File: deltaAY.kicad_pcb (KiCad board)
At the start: 2 copper layers, 97 x 61.4 mm, 18 parts, among them J1 SNP, J2 Jack_3.5mm_5pin, U1 М555ЛН1 (SN74LS04), U2 К555ТМ2 (SN74LS74), U3 К555ЛЛ1 (SN74LS32), U4 К555ЛЕ1 (SN74LS02), Y1 3.579545Mhz

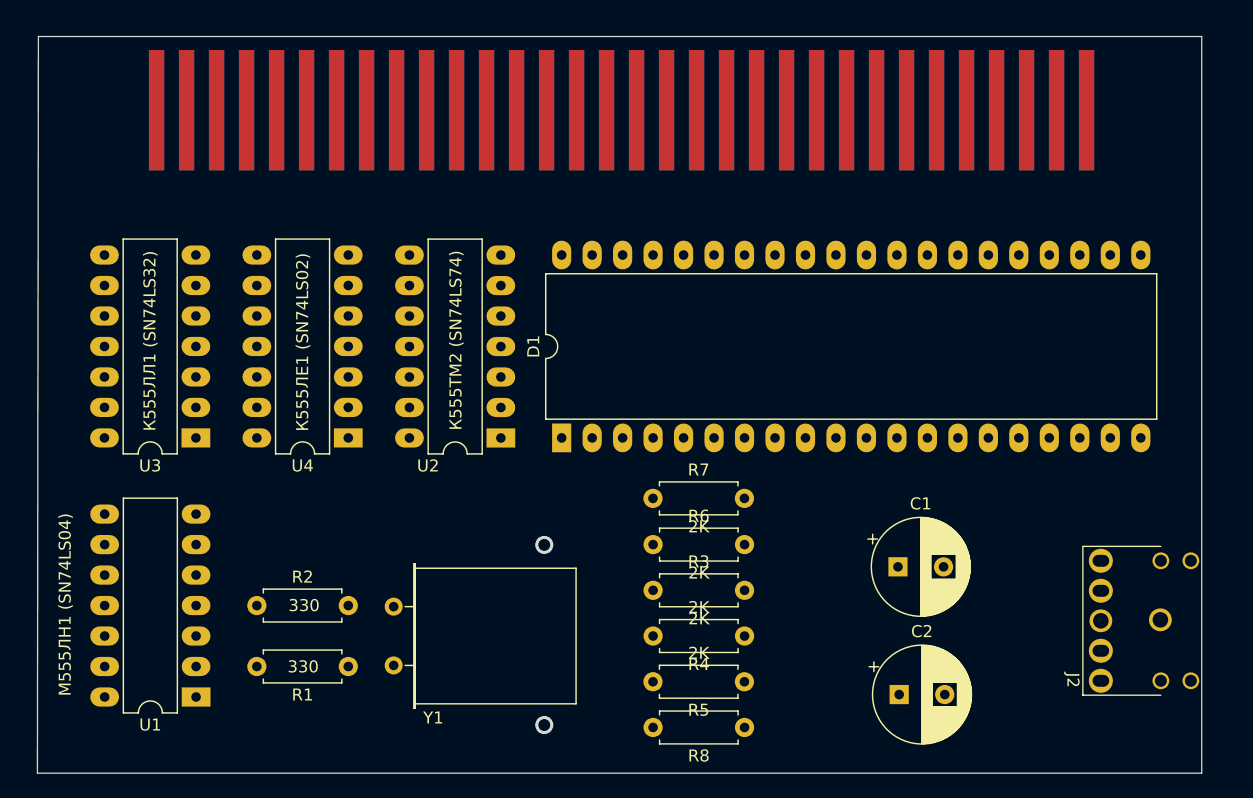
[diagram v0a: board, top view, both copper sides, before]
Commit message: Update 19072023
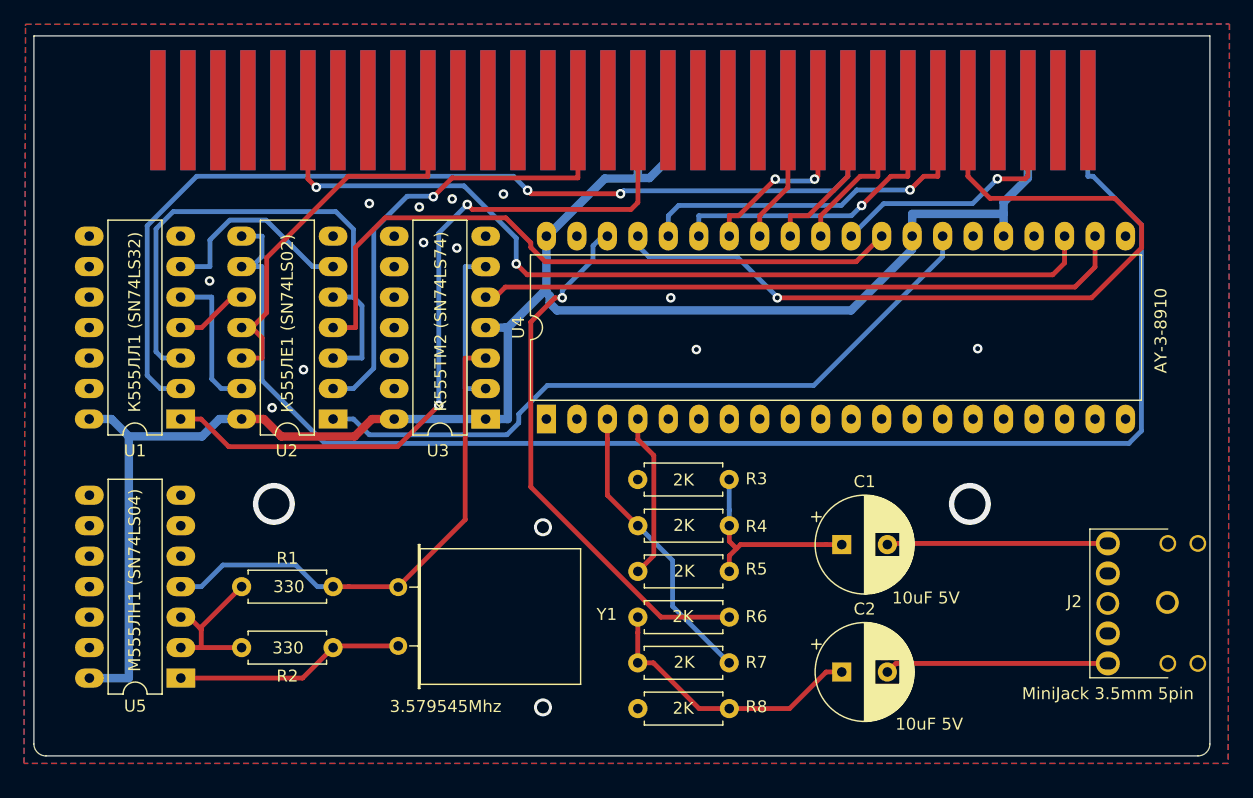
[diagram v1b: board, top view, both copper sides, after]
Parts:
- J1: value SNP -> СНП59-96
- J2: value Jack_3.5mm_5pin -> MiniJack 3.5mm 5pin
- U4: renamed from D1; value ~ -> AY-3-8910
- moved C2 5.14 mm to (117.3, 83.0)
- moved C1 5.04 mm to (117.3, 72.4)
- moved R3 2.02 mm to (100.3, 67.0)
- moved U5 2.02 mm to (62.2, 83.5)
- moved U3 2.02 mm to (87.6, 61.9)
- moved U4 2.02 mm to (92.7, 61.9)
- moved R6 2.02 mm to (108.0, 78.4)
- moved U1 2.02 mm to (62.2, 61.9)
- moved U2 2.02 mm to (74.9, 61.9)
- moved R1 2.02 mm to (67.3, 75.9)
- moved R2 2.02 mm to (74.9, 81.0)
- moved R4 2.02 mm to (100.3, 70.8)
- moved R5 2.02 mm to (100.3, 74.6)
- moved R7 2.02 mm to (107.9, 82.2)
- moved R8 2.02 mm to (108.0, 86.1)
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- renumbered R2 to R1, R1 to R2, R7 to R3, R6 to R4, R3 to R5, R4 to R6, R5 to R7, U3 to U1, U4 to U2, U2 to U3, U1 to U5
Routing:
- net +5V: track 0.00 -> 157.5 mm
- net A14: track 0.00 -> 120.5 mm
- net A1: track 0.00 -> 82.5 mm, vias 0 -> 2
- net RESET: track 0.00 -> 76.1 mm, vias 0 -> 2
- net DA0: track 0.00 -> 69.9 mm, vias 0 -> 1
- net IORQ: track 0.00 -> 63.9 mm, vias 0 -> 2
- net AY27: track 0.00 -> 59.6 mm
- net AY29: track 0.00 -> 56.1 mm
- net AY22: track 0.00 -> 54.4 mm
- net Net-(U3-Pad3): track 0.00 -> 45.3 mm
- net AY_C: track 0.00 -> 45.2 mm, vias 0 -> 1
- net Net-(U2A-C): track 0.00 -> 42.7 mm
- net WR: track 0.00 -> 40.1 mm, vias 0 -> 1
- net M1: track 0.00 -> 33.5 mm
- net DA1: track 0.00 -> 31.0 mm, vias 0 -> 1
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- added copper zone on B.Cu, net GND
- added copper zone on F.Cu, net GND
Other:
- board size 97 x 61.4 mm -> 98 x 60 mm
